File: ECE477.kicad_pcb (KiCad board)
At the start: 2 copper layers, 88.9 x 88.9 mm, 55 parts, among them IC1 LP3852EMP-3.3_NOPB, IC2 BQ29330DBT, J1 P7805-2000-S, J10 Conn_01x01_Male, J11 Conn_01x01_Male, J2 Conn_01x05_Male, J3 Conn_01x05_Male, J4 Conn_01x05_Male, J5 Conn_01x05_Male, J6 Conn_01x05_Male, J7 Conn_01x05_Male, J8 Conn_01x05_Male, J9 Conn_01x01_Male, SW1 SW_Push_Dual, U1 STM32H7_LQFP144_T2

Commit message: naming
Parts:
- J10: value Conn_01x01_Male -> USART3
- J11: value Conn_01x01_Male -> USART1
- J9: value Conn_01x01_Male -> USART6

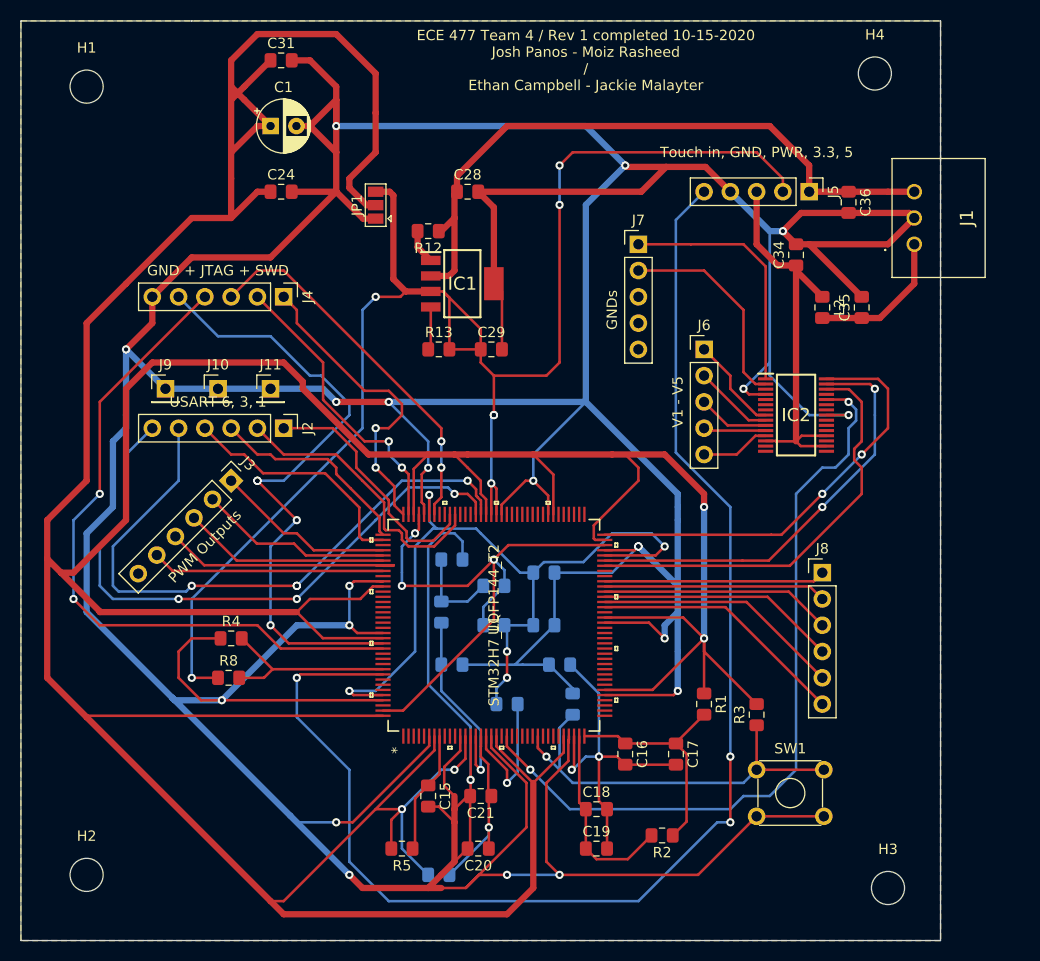
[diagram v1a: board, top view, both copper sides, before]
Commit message: Major change
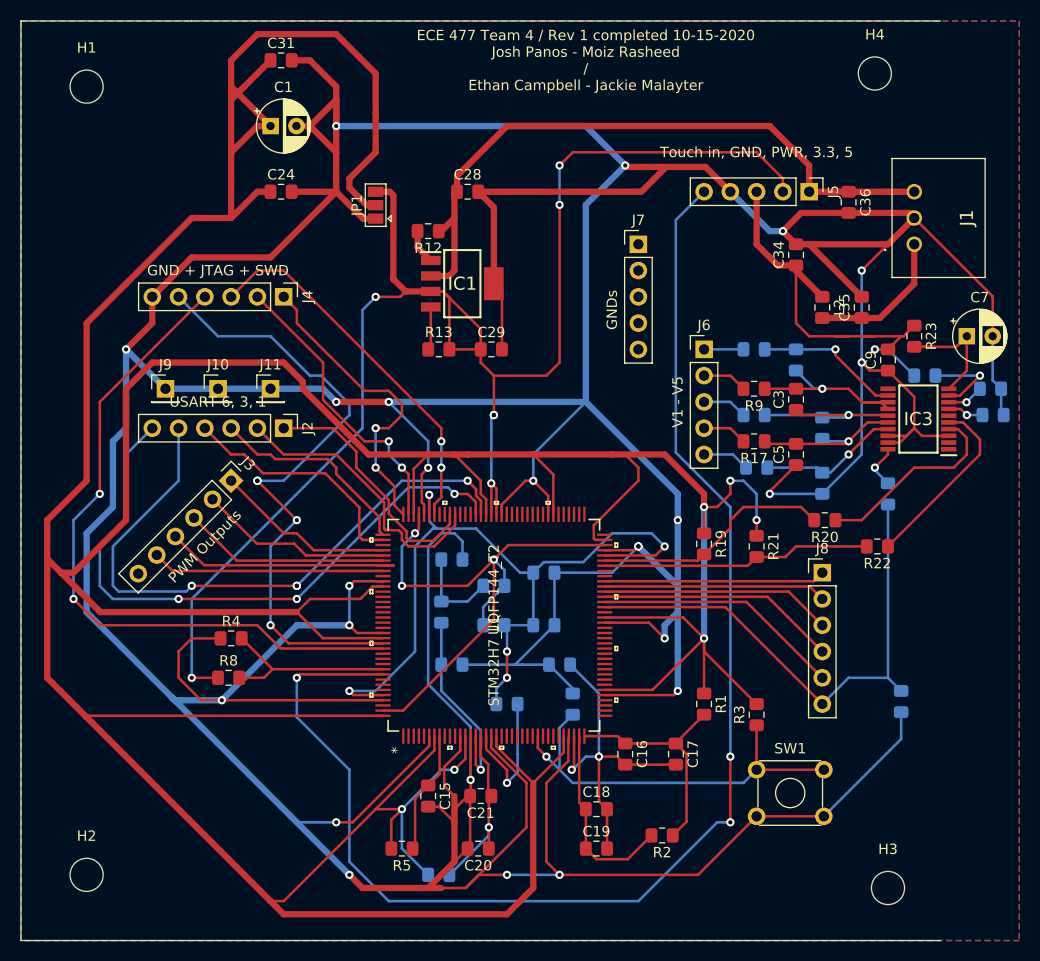
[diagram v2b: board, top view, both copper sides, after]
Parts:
- removed IC2: BQ29330DBT, SamacSys_Parts:SOP50P640X120-30N
- added C10: 1uF, Capacitor_SMD:C_0805_2012Metric_Pad1.15x1.40mm_HandSolder, B.Cu at (246.1, 83.8)
- added C2: 1uF, Capacitor_SMD:C_0805_2012Metric_Pad1.15x1.40mm_HandSolder, B.Cu at (227.3, 81.0)
- added C3: 1uF, Capacitor_SMD:C_0805_2012Metric_Pad1.15x1.40mm_HandSolder, F.Cu at (227.3, 84.8)
- added C4: 1uF, Capacitor_SMD:C_0805_2012Metric_Pad1.15x1.40mm_HandSolder, B.Cu at (229.9, 87.6)
- added C5: 1uF, Capacitor_SMD:C_0805_2012Metric_Pad1.15x1.40mm_HandSolder, F.Cu at (227.3, 90.2)
- added C6: 1uF, Capacitor_SMD:C_0805_2012Metric_Pad1.15x1.40mm_HandSolder, B.Cu at (229.9, 93.0)
- added C7: 10uF, Capacitor_THT:CP_Radial_D5.0mm_P2.50mm, F.Cu at (243.8, 78.7)
- added C8: 1uF, Capacitor_SMD:C_0805_2012Metric_Pad1.15x1.40mm_HandSolder, B.Cu at (246.4, 86.4)
- added C9: 1uF, Capacitor_SMD:C_0805_2012Metric_Pad1.15x1.40mm_HandSolder, F.Cu at (236.2, 81.0)
- added IC3: BQ7692006PWR, SamacSys_Parts:SOP65P640X120-20N, F.Cu at (239.2, 86.7)
- added R15: 100, Resistor_SMD:R_0805_2012Metric_Pad1.15x1.40mm_HandSolder, B.Cu at (223.3, 80.0)
- added R16: 100, Resistor_SMD:R_0805_2012Metric_Pad1.15x1.40mm_HandSolder, B.Cu at (223.3, 86.4)
- added R17: 100, Resistor_SMD:R_0805_2012Metric_Pad1.15x1.40mm_HandSolder, F.Cu at (223.3, 88.9)
- added R18: 100, Resistor_SMD:R_0805_2012Metric_Pad1.15x1.40mm_HandSolder, B.Cu at (223.5, 91.4)
- added R19: 1k, Resistor_SMD:R_0805_2012Metric_Pad1.15x1.40mm_HandSolder, F.Cu at (218.4, 98.8)
- added R20: 0R, Resistor_SMD:R_0805_2012Metric_Pad1.15x1.40mm_HandSolder, F.Cu at (230.1, 96.5)
- added R21: 1k, Resistor_SMD:R_0805_2012Metric_Pad1.15x1.40mm_HandSolder, F.Cu at (223.5, 99.1)
- added R22: 0R, Resistor_SMD:R_0805_2012Metric_Pad1.15x1.40mm_HandSolder, F.Cu at (235.2, 99.1)
- added R23: 100, Resistor_SMD:R_0805_2012Metric_Pad1.15x1.40mm_HandSolder, F.Cu at (238.8, 78.7)
- added R24: 0R, Resistor_SMD:R_0805_2012Metric_Pad1.15x1.40mm_HandSolder, B.Cu at (239.8, 82.5)
- added R25: 0R, Resistor_SMD:R_0805_2012Metric_Pad1.15x1.40mm_HandSolder, B.Cu at (236.2, 94.0)
- added R26: 1M, Resistor_SMD:R_0805_2012Metric_Pad1.15x1.40mm_HandSolder, B.Cu at (237.5, 114.1)
- added R9: 100, Resistor_SMD:R_0805_2012Metric_Pad1.15x1.40mm_HandSolder, F.Cu at (223.3, 83.8)
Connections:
- U1 pad 21: CLK -> Net-(U1-Pad21)
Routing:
- net CLK: track 74.3 -> 0.00 mm, vias 2 -> 0
- net GND: track 691.6 -> 752.4 mm, vias 22 -> 24
- net I2C2_SMBA: track 41.8 -> 0.00 mm, vias 2 -> 0
- net PIN1: track 24.9 -> 50.9 mm
- net CELL-: track 24.1 -> 0.00 mm
- net CELL+: track 20.4 -> 0.00 mm
- net SDA_1: track 0.00 -> 19.0 mm
- net cell_3: track 0.00 -> 18.5 mm, vias 0 -> 1
- net SCL_1: track 0.00 -> 17.7 mm
- net I2C2_SDA: track 41.6 -> 23.9 mm, vias 2 -> 0
- net cell_2: track 0.00 -> 17.4 mm, vias 0 -> 1
- net cell_1: track 0.00 -> 15.5 mm, vias 0 -> 1
- net I2C2_SCL: track 41.1 -> 26.1 mm
- net cell_pwr: track 0.00 -> 14.1 mm, vias 0 -> 1
- net VDD_MCU: track 489.0 -> 503.0 mm, vias 4 -> 6
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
